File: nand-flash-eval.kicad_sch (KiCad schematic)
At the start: 1 part, among them U1 TC58BVG0S3HTA00

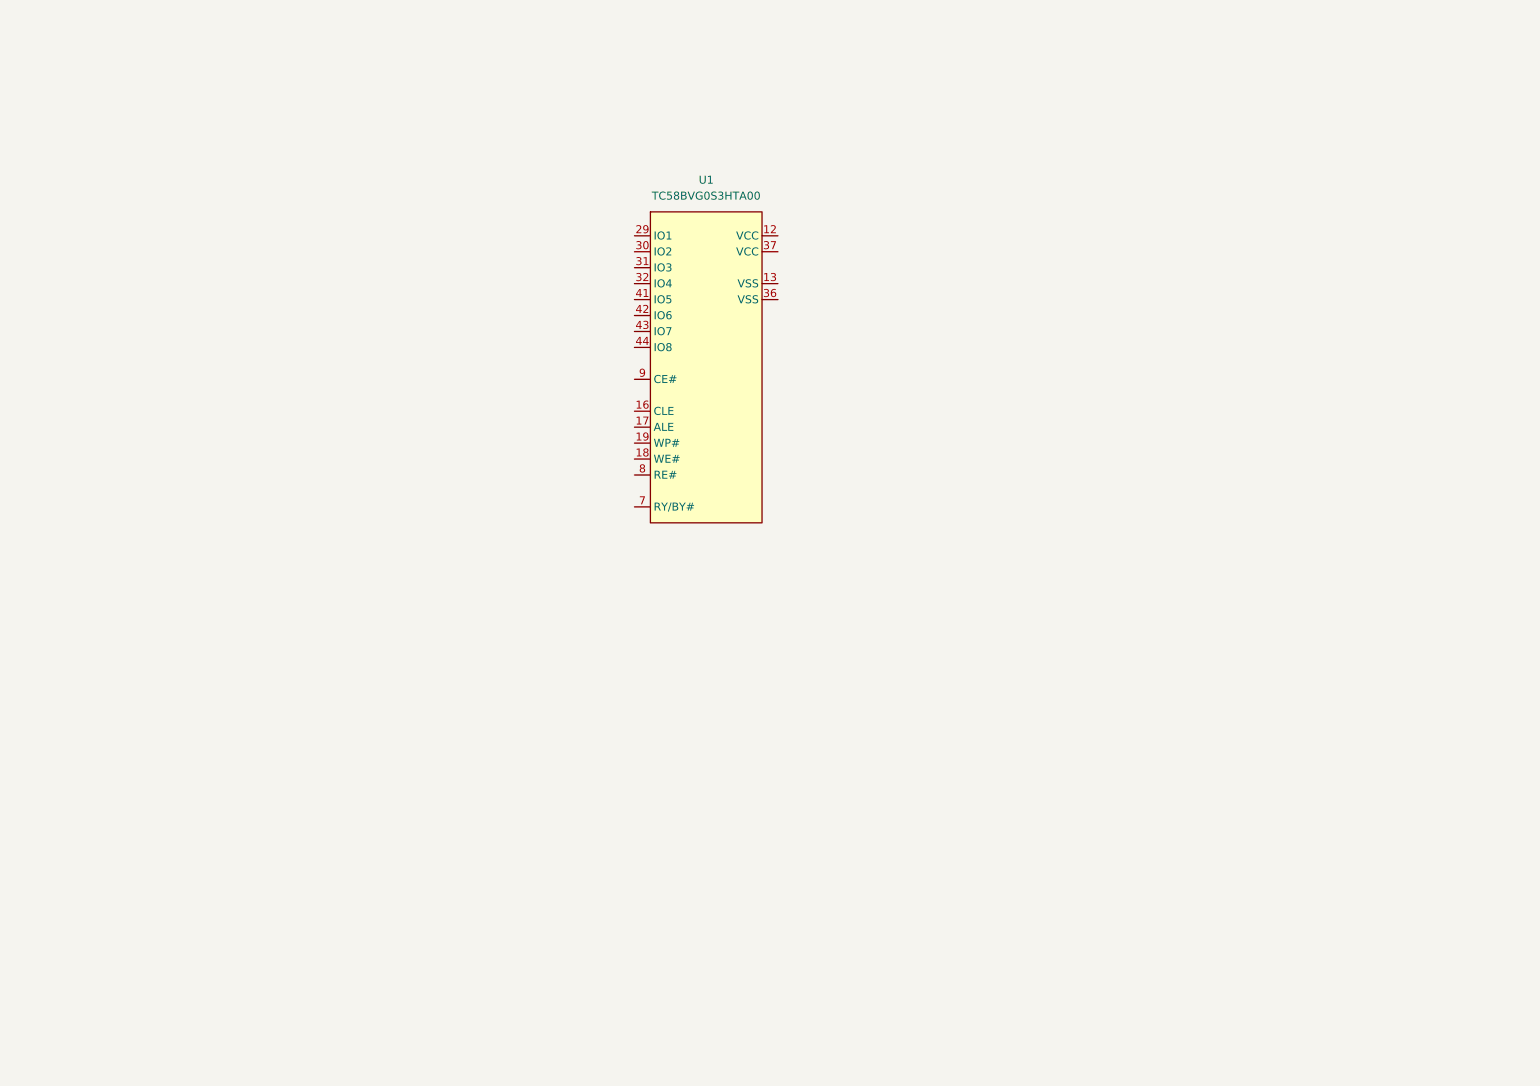
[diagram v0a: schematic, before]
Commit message: feat: 大体書いた
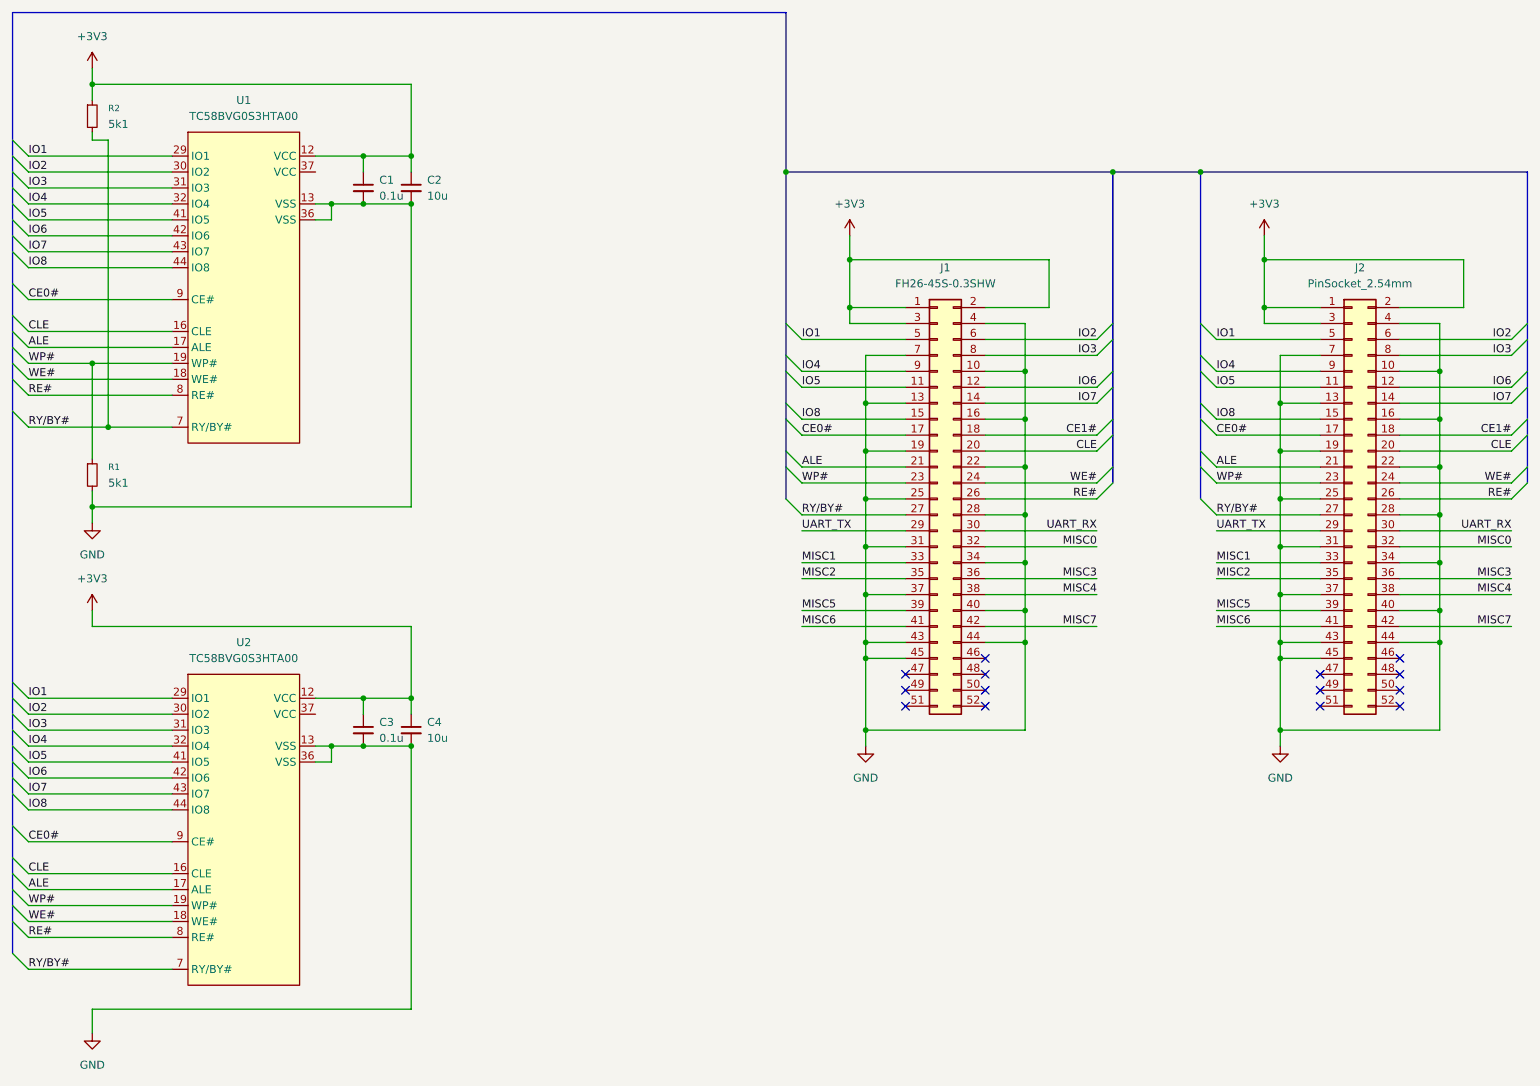
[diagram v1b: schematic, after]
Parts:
- added C1, C3: 0.1u, Capacitor_SMD:C_0402_1005Metric, symbol Device:C_Small
- added C2, C4: 10u, Capacitor_SMD:C_0402_1005Metric, symbol Device:C_Small
- added J1: FH26-45S-0.3SHW, Connector_FFC-FPC:Hirose_FH26-45S-0.3SHW_2Rows-45Pins-1MP_P0.60mm_Horizontal, symbol Connector_Generic:Conn_02x26_Odd_Even
- added J2: PinSocket_2.54mm, Connector_PinSocket_2.54mm:PinSocket_2x25_P2.54mm_Vertical, symbol Connector_Generic:Conn_02x26_Odd_Even
- added R1, R2: 5k1, symbol Device:R_Small
- added U2: TC58BVG0S3HTA00, Package_SO:TSOP-I-48_18.4x12mm_P0.5mm, symbol nand-flash-eval:TC58BVG0S3HTA00
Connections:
- net +3V3: now reaches U1.12 (VCC)
- net +3V3: now also C1.1, C2.1, C3.1, C4.1, J1.1 (Pin_1), J1.2 (Pin_2), J1.3 (Pin_3), J2.1 (Pin_1), J2.2 (Pin_2), J2.3 (Pin_3), R2.1, U2.12 (VCC)
- net GND: now reaches U1.13 (VSS)
- net GND: now also U1.36 (VSS), C1.2, C2.2, C3.2, C4.2, J1.10 (Pin_10), J1.13 (Pin_13), J1.16 (Pin_16), J1.19 (Pin_19), J1.22 (Pin_22), J1.25 (Pin_25), J1.28 (Pin_28), J1.31 (Pin_31), J1.34 (Pin_34), J1.37 (Pin_37), J1.4 (Pin_4), J1.40 (Pin_40), J1.43 (Pin_43), J1.44 (Pin_44), J1.45 (Pin_45), J1.7 (Pin_7), J2.10 (Pin_10), J2.13 (Pin_13), J2.16 (Pin_16), J2.19 (Pin_19), J2.22 (Pin_22), J2.25 (Pin_25), J2.28 (Pin_28), J2.31 (Pin_31), J2.34 (Pin_34), J2.37 (Pin_37), J2.4 (Pin_4), J2.40 (Pin_40), J2.43 (Pin_43), J2.44 (Pin_44), J2.45 (Pin_45), J2.7 (Pin_7), R1.2, U2.13 (VSS), U2.36 (VSS)
- net CLE: now reaches U1.16 (CLE)
- net CLE: now also J1.20 (Pin_20), J2.20 (Pin_20), U2.16 (CLE)
- net ALE: now reaches U1.17 (ALE)
- net ALE: now also J1.21 (Pin_21), J2.21 (Pin_21), U2.17 (ALE)
- net WE#: now reaches U1.18 (WE#)
- net WE#: now also J1.24 (Pin_24), J2.24 (Pin_24), U2.18 (WE#)
- net WP#: now reaches U1.19 (WP#)
- net WP#: now also J1.23 (Pin_23), J2.23 (Pin_23), R1.1, U2.19 (WP#)
- net IO1: now reaches U1.29 (IO1)
- net IO1: now also J1.5 (Pin_5), J2.5 (Pin_5), U2.29 (IO1)
- net IO2: now reaches U1.30 (IO2)
- net IO2: now also J1.6 (Pin_6), J2.6 (Pin_6), U2.30 (IO2)
- net IO3: now reaches U1.31 (IO3)
- net IO3: now also J1.8 (Pin_8), J2.8 (Pin_8), U2.31 (IO3)
- net IO4: now reaches U1.32 (IO4)
- net IO4: now also J1.9 (Pin_9), J2.9 (Pin_9), U2.32 (IO4)
- net IO5: now reaches U1.41 (IO5)
- net IO5: now also J1.11 (Pin_11), J2.11 (Pin_11), U2.41 (IO5)
- net IO6: now reaches U1.42 (IO6)
- net IO6: now also J1.12 (Pin_12), J2.12 (Pin_12), U2.42 (IO6)
- net IO7: now reaches U1.43 (IO7)
- net IO7: now also J1.14 (Pin_14), J2.14 (Pin_14), U2.43 (IO7)
- net IO8: now reaches U1.44 (IO8)
- net IO8: now also J1.15 (Pin_15), J2.15 (Pin_15), U2.44 (IO8)
- net RY/BY#: now reaches U1.7 (RY/BY#)
- net RY/BY#: now also J1.27 (Pin_27), J2.27 (Pin_27), R2.2, U2.7 (RY/BY#)
- net RE#: now reaches U1.8 (RE#)
- net RE#: now also J1.26 (Pin_26), J2.26 (Pin_26), U2.8 (RE#)
- net CE0#: now reaches U1.9 (CE#)
- net CE0#: now also J1.17 (Pin_17), J2.17 (Pin_17), U2.9 (CE#)
- new net CE1#: J1.18 (Pin_18), J2.18 (Pin_18)
- new net MISC0: J1.32 (Pin_32), J2.32 (Pin_32)
- new net MISC1: J1.33 (Pin_33), J2.33 (Pin_33)
- new net MISC2: J1.35 (Pin_35), J2.35 (Pin_35)
- new net MISC3: J1.36 (Pin_36), J2.36 (Pin_36)
- new net MISC4: J1.38 (Pin_38), J2.38 (Pin_38)
- new net MISC5: J1.39 (Pin_39), J2.39 (Pin_39)
- new net MISC6: J1.41 (Pin_41), J2.41 (Pin_41)
- new net MISC7: J1.42 (Pin_42), J2.42 (Pin_42)
- new net UART_RX: J1.30 (Pin_30), J2.30 (Pin_30)
- new net UART_TX: J1.29 (Pin_29), J2.29 (Pin_29)
- no-connect marks 0 -> 14
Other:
- moved on the sheet: U1
